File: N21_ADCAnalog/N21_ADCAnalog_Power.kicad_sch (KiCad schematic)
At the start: 11 parts

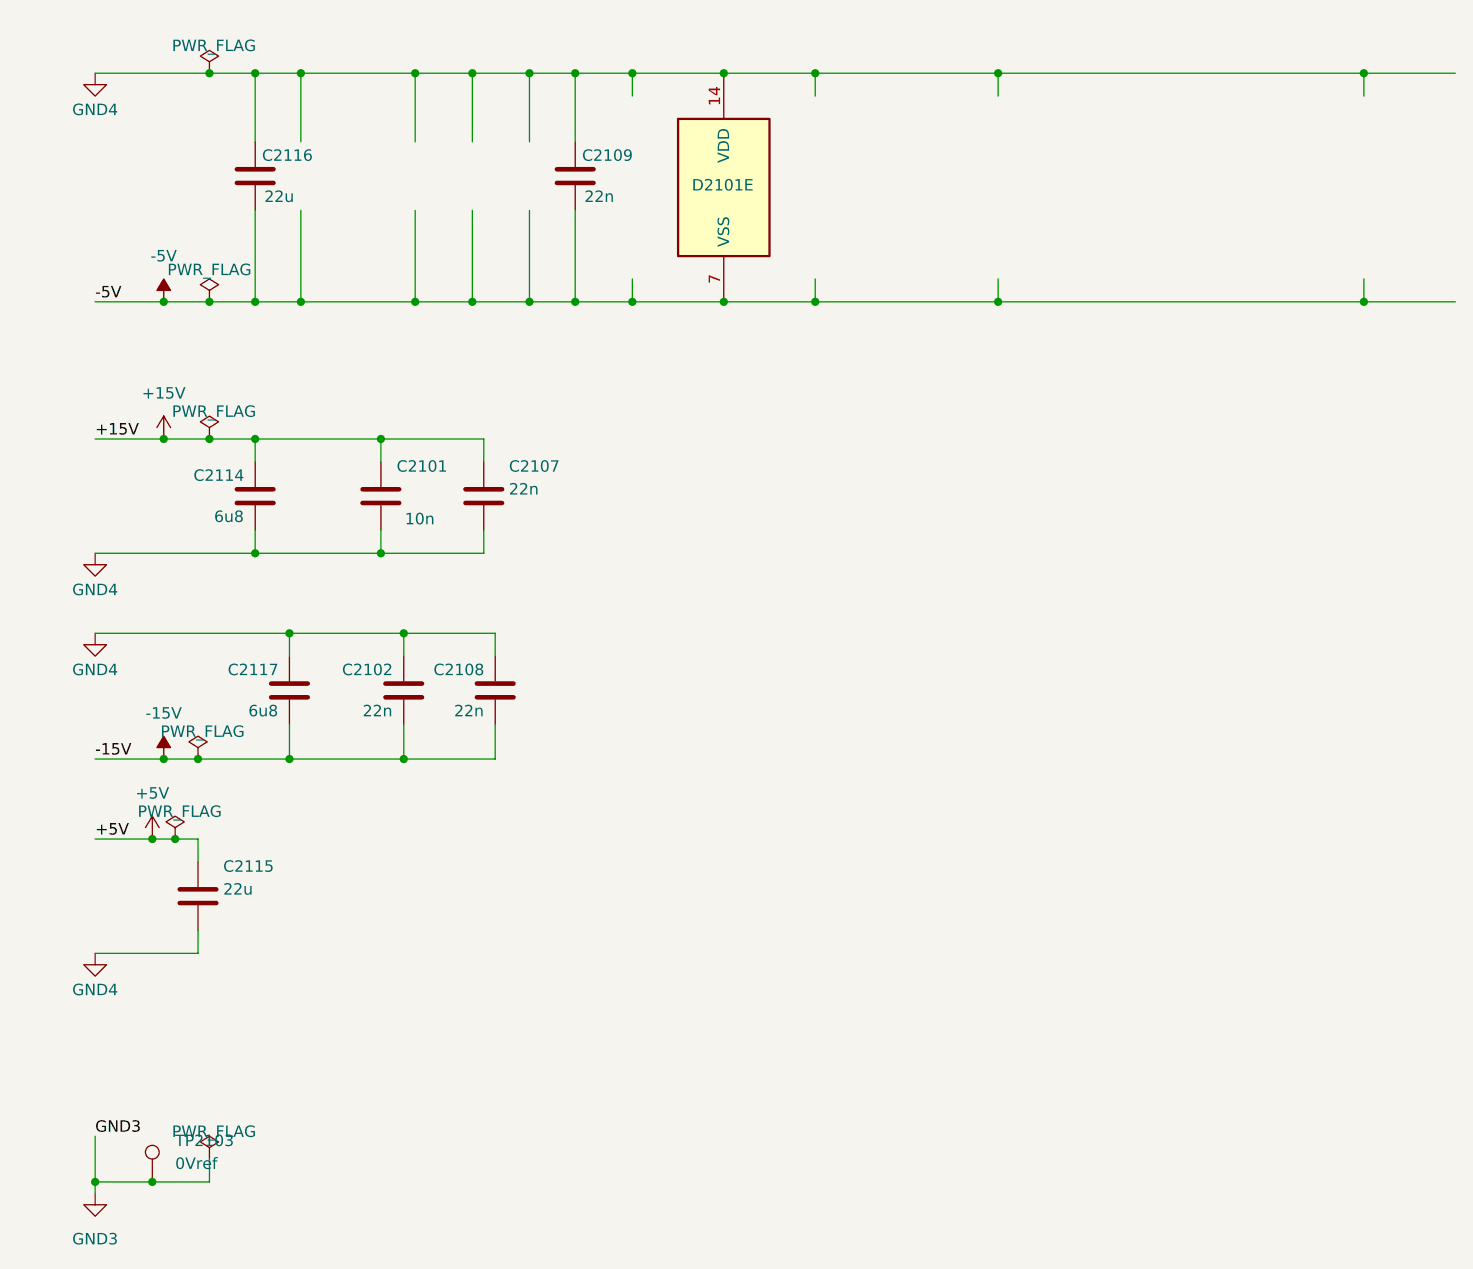
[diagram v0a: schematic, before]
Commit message: Updates, add N25
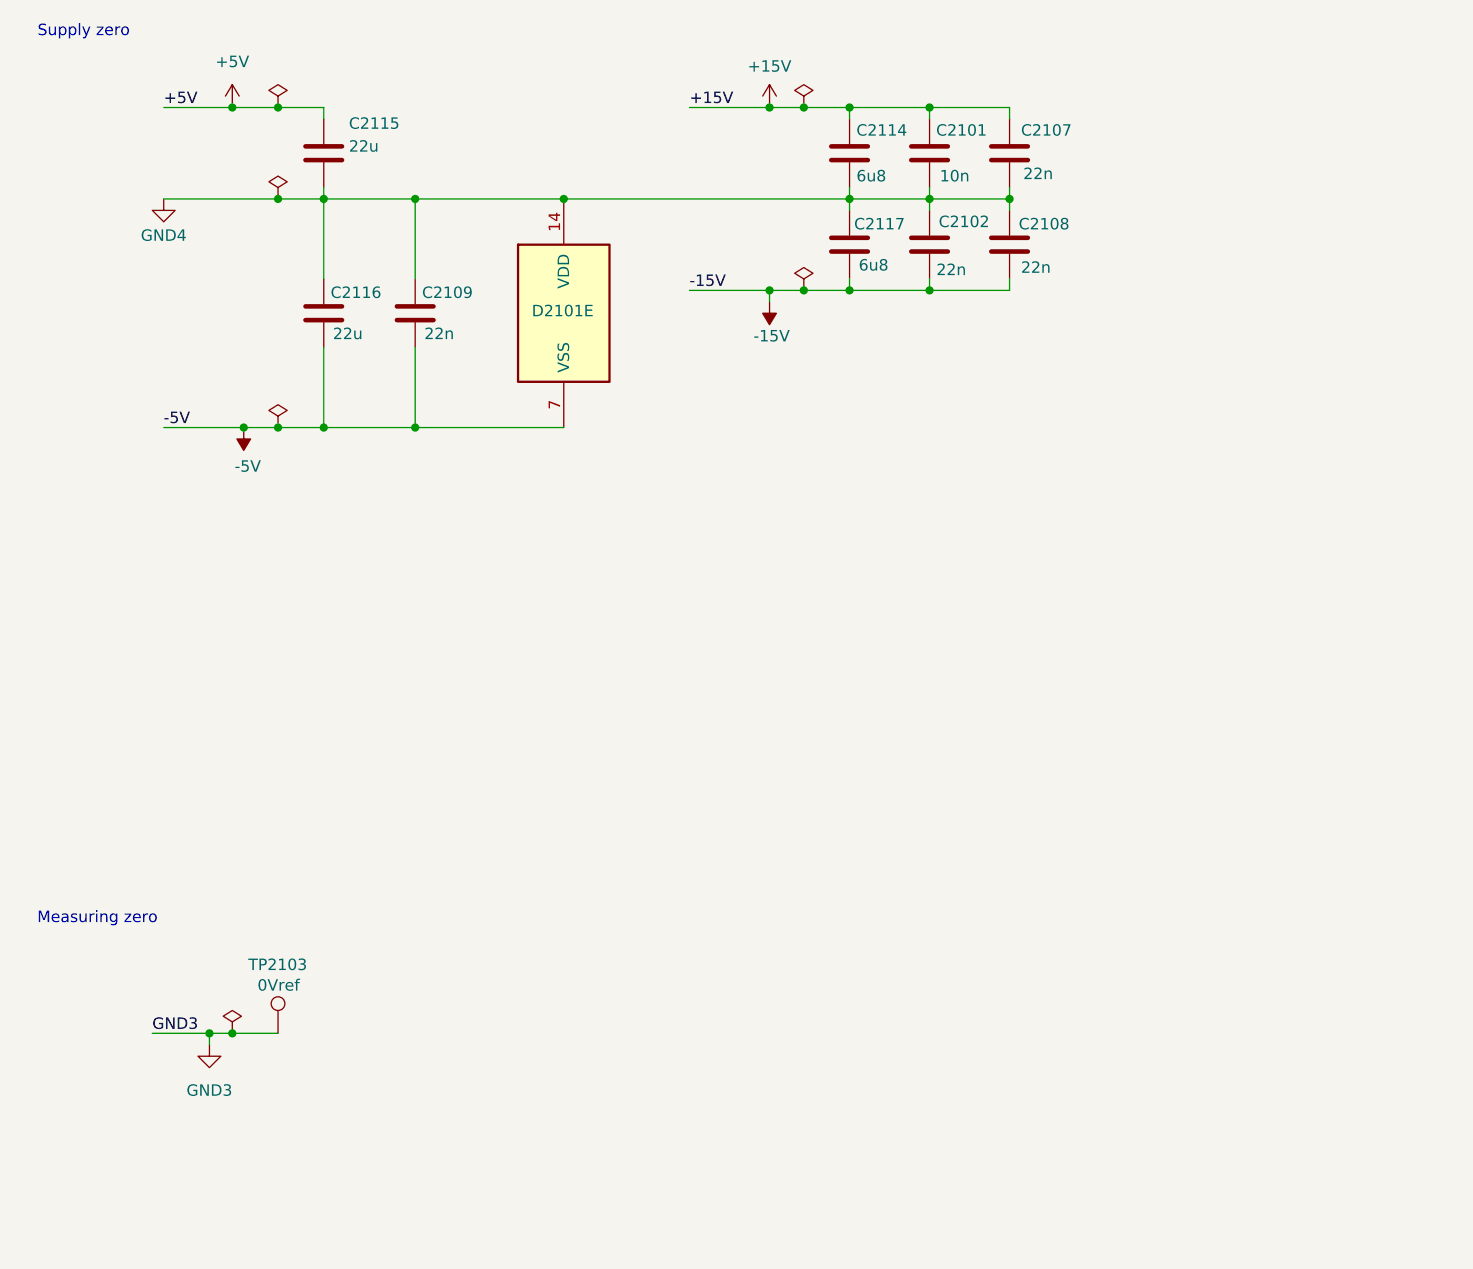
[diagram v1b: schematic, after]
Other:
- note added: "Measuring zero"
- note added: "Supply zero"
- moved on the sheet: C2101, C2102, C2107, C2108, C2109, C2114, C2115, C2116, C2117, D2101E, TP2103
